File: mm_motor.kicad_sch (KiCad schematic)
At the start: 1 part, among them M1 N20_encoder

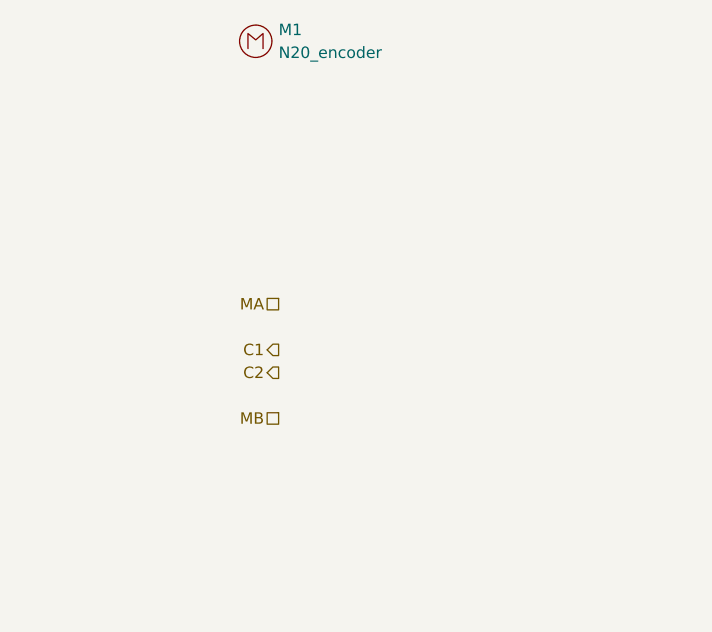
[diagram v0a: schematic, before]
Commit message: fin tp2
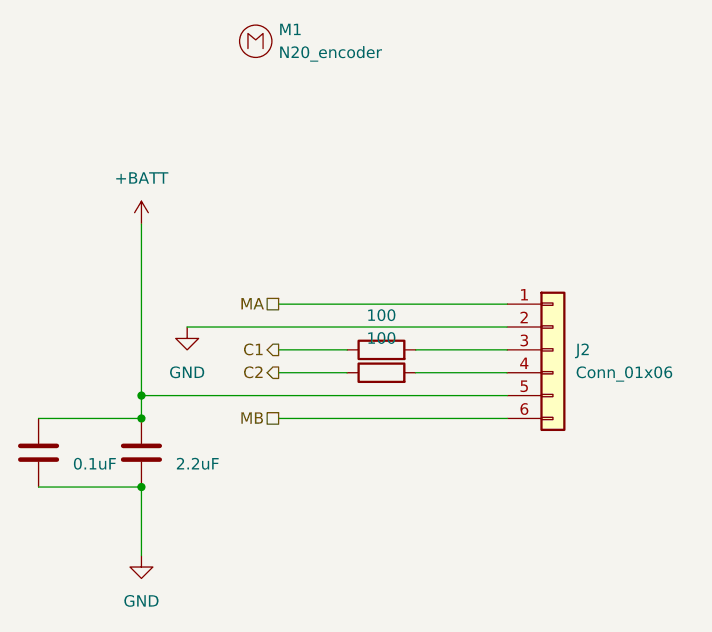
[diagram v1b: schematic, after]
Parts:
- added C15: 2.2uF, Capacitor_SMD:C_0603_1608Metric, symbol minimouse:C
- added C17: 0.1uF, Capacitor_SMD:C_0603_1608Metric, symbol minimouse:C
- added J2: Conn_01x06, Connector_PinHeader_2.54mm:PinHeader_1x06_P2.54mm_Vertical, symbol Connector_Generic:Conn_01x06
- added R19 (x2): 100, Resistor_SMD:R_0603_1608Metric, symbol minimouse:R
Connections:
- net C1: now also R19.1
- net C2: now also R19.1
- net MA: now also J2.1 (Pin_1)
- net MB: now also J2.6 (Pin_6)
- new net: J2.3 (Pin_3), R19.2
- new net: J2.4 (Pin_4), R19.2
- new net +BATT: C15.1, C17.1, J2.5 (Pin_5)
- new net GND: C15.2, C17.2, J2.2 (Pin_2)
